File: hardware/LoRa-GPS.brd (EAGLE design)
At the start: 50.8 x 17.8 mm, 30 parts, among them J1 10118193-0001LF, Q1 IRLML6402, U1 MCP1703-3302E/CB, Y1 CRYSTAL.ABS07

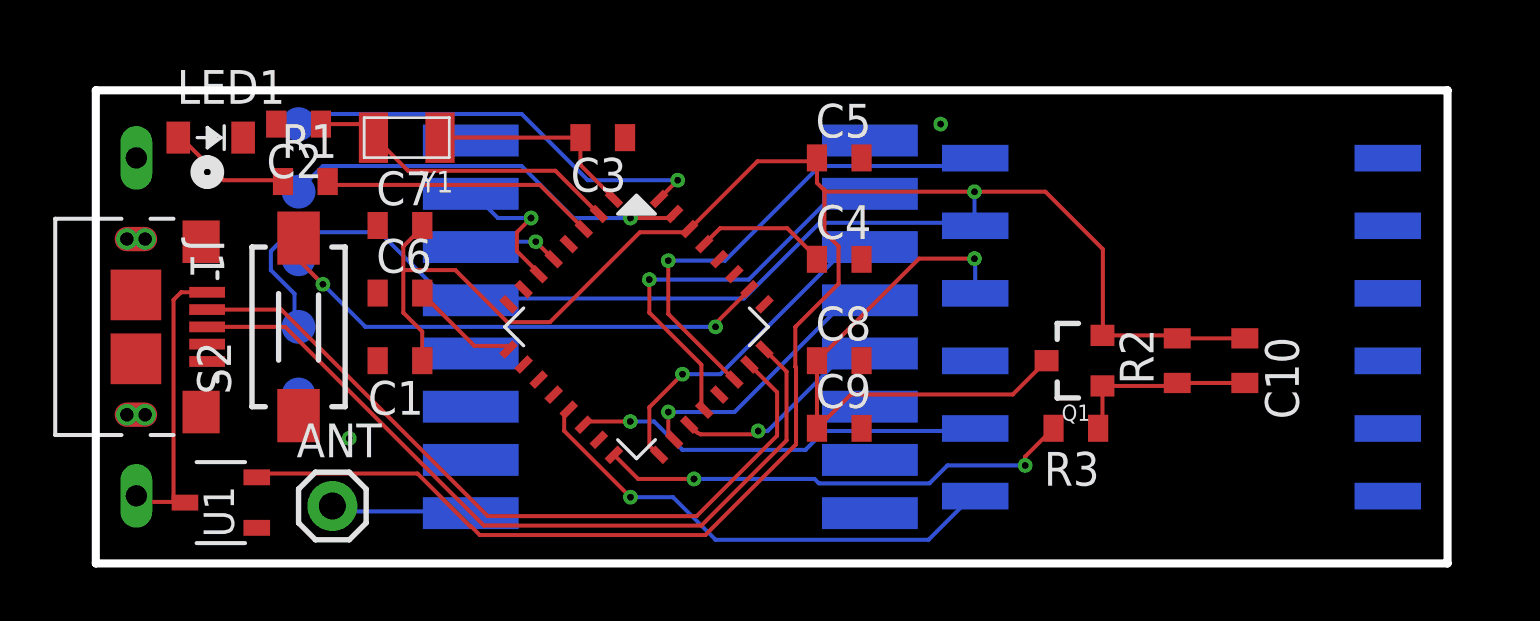
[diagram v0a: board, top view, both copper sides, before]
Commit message: ripup
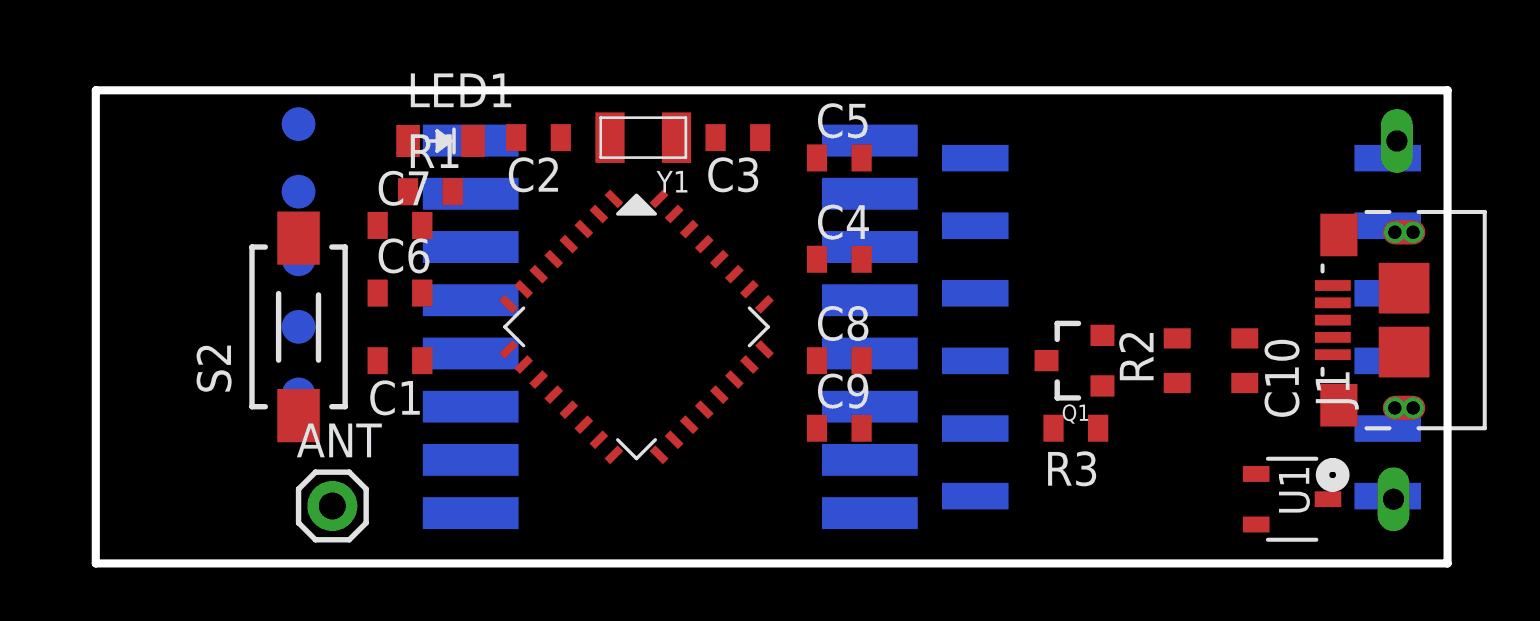
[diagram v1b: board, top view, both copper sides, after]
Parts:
- moved J1 47.6 mm to (49.1, 9.14), turned to 90 degrees
- moved JP2 47.4 mm to (48.9, 15.9)
- moved JP1 47.2 mm to (48.8, 2.41)
- moved U1 40.3 mm to (45.0, 2.41), turned to 270 degrees
- moved C2 9.03 mm to (16.6, 16.0)
- moved Y1 8.89 mm to (20.6, 16.0)
- moved LED1 8.64 mm to (13.0, 15.9)
- moved C3 5.08 mm to (24.1, 16.0)
- moved R1 4.71 mm to (12.6, 14.0)
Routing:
- net VCC: track 112.8 -> 0.00 mm, vias 1 -> 0
- net D+: track 30.0 -> 0.00 mm
- net D-: track 29.0 -> 0.00 mm
- net N$7: track 21.0 -> 0.00 mm, vias 1 -> 0
- net RESET: track 20.8 -> 0.00 mm, vias 2 -> 0
- net TX: track 18.7 -> 0.00 mm, vias 1 -> 0
- net D21: track 18.6 -> 0.00 mm, vias 1 -> 0
- net GPSPOWER: track 18.0 -> 0.00 mm, vias 2 -> 0
- net SWDIO: track 16.4 -> 0.00 mm, vias 1 -> 0
- net RX: track 15.5 -> 0.00 mm, vias 1 -> 0
- net SWCLK: track 15.5 -> 0.00 mm, vias 1 -> 0
- net MISO: track 15.4 -> 0.00 mm, vias 1 -> 0
- net MOSI: track 12.8 -> 0.00 mm, vias 1 -> 0
- net N$2: track 11.8 -> 0.00 mm
- net VIN: track 10.9 -> 0.00 mm
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
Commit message: Revert "ripup"
This reverts commit 834d71edbbdf070d64fbb4b16cb78b1eed2d9a3e.
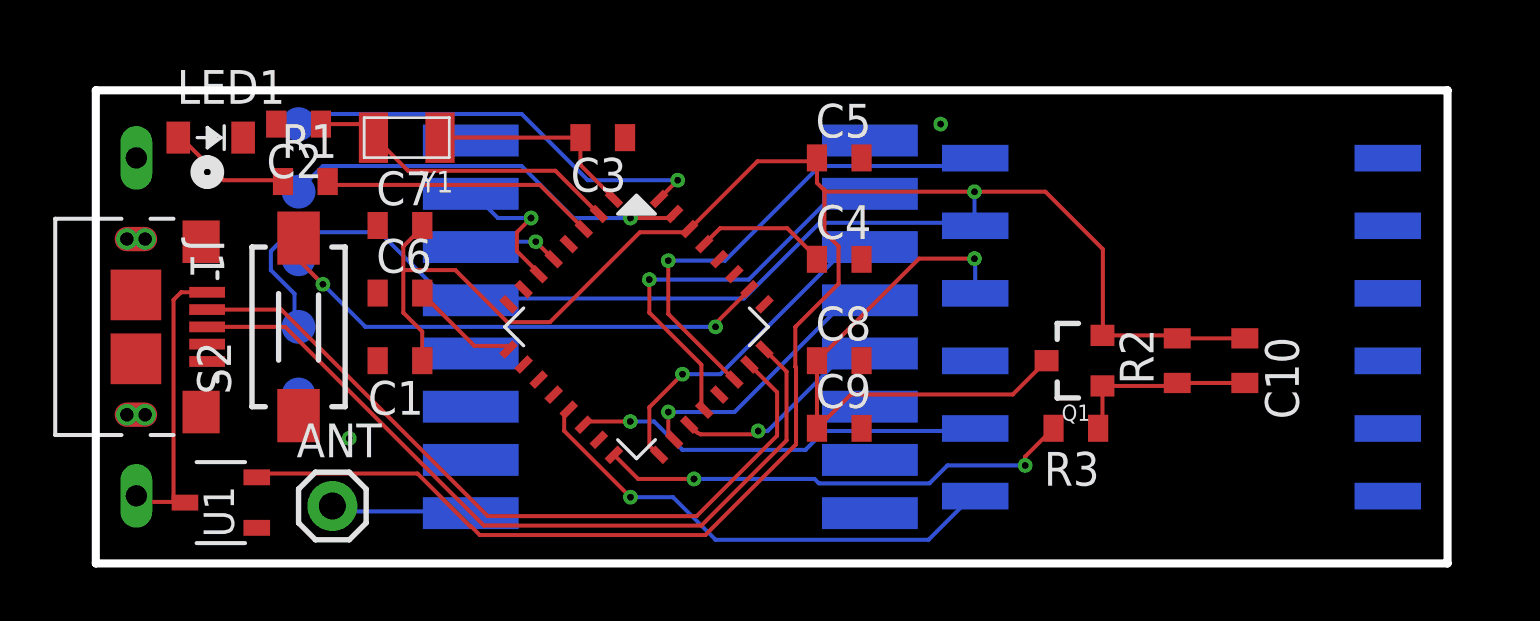
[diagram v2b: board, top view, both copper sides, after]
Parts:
- moved J1 47.6 mm to (1.52, 8.89), turned to 270 degrees
- moved JP2 47.4 mm to (1.52, 15.2)
- moved JP1 47.2 mm to (1.52, 2.54)
- moved U1 40.3 mm to (4.70, 2.29), turned to 90 degrees
- moved C2 9.03 mm to (7.62, 16.5)
- moved Y1 8.89 mm to (11.7, 16.0)
- moved LED1 8.64 mm to (4.32, 16.0)
- moved C3 5.08 mm to (19.1, 16.0)
- moved R1 4.71 mm to (7.87, 14.4)
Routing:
- net VCC: track 0.00 -> 112.8 mm, vias 0 -> 1
- net D+: track 0.00 -> 30.0 mm
- net D-: track 0.00 -> 29.0 mm
- net N$7: track 0.00 -> 21.0 mm, vias 0 -> 1
- net RESET: track 0.00 -> 20.8 mm, vias 0 -> 2
- net TX: track 0.00 -> 18.7 mm, vias 0 -> 1
- net D21: track 0.00 -> 18.6 mm, vias 0 -> 1
- net GPSPOWER: track 0.00 -> 18.0 mm, vias 0 -> 2
- net SWDIO: track 0.00 -> 16.4 mm, vias 0 -> 1
- net RX: track 0.00 -> 15.5 mm, vias 0 -> 1
- net SWCLK: track 0.00 -> 15.5 mm, vias 0 -> 1
- net MISO: track 0.00 -> 15.4 mm, vias 0 -> 1
- net MOSI: track 0.00 -> 12.8 mm, vias 0 -> 1
- net N$2: track 0.00 -> 11.8 mm
- net VIN: track 0.00 -> 10.9 mm
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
